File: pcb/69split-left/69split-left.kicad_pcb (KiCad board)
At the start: 2 copper layers, 157.5 x 108.9 mm, 96 parts, among them J1 USB_C_Receptacle_USB2.0_16P, J2 Conn_02x03_Odd_Even, J3 USB_C_Receptacle_USB2.0_16P, J4 Conn_01x09_Socket, SW1 SW_Push, SW10 SW_Push, SW11 SW_Push, SW12 SW_Push, SW13 SW_Push, SW14 SW_Push, SW15 SW_Push, SW16 SW_Push, SW17 SW_Push, SW18 SW_Push, SW19 SW_Push, SW2 SW_Push, SW20 SW_Push, SW21 SW_Push, SW22 SW_Push, SW23 SW_Push, SW24 SW_Push, SW25 SW_Push, SW26 SW_Push, SW27 SW_Push, SW28 SW_Push, SW29 SW_Push, SW3 SW_Push, SW30 SW_Push, SW31 SW_Push, SW32 SW_SPDT, SW4 SW_Push, SW5 SW_Push, SW6 SW_Push, SW7 SW_Push, SW8 SW_Push, SW9 SW_Push, U1 ATmega32U4-AU, U2 TLV76133DCY, U3 TPD2E2U06DCK, Y1 Crystal

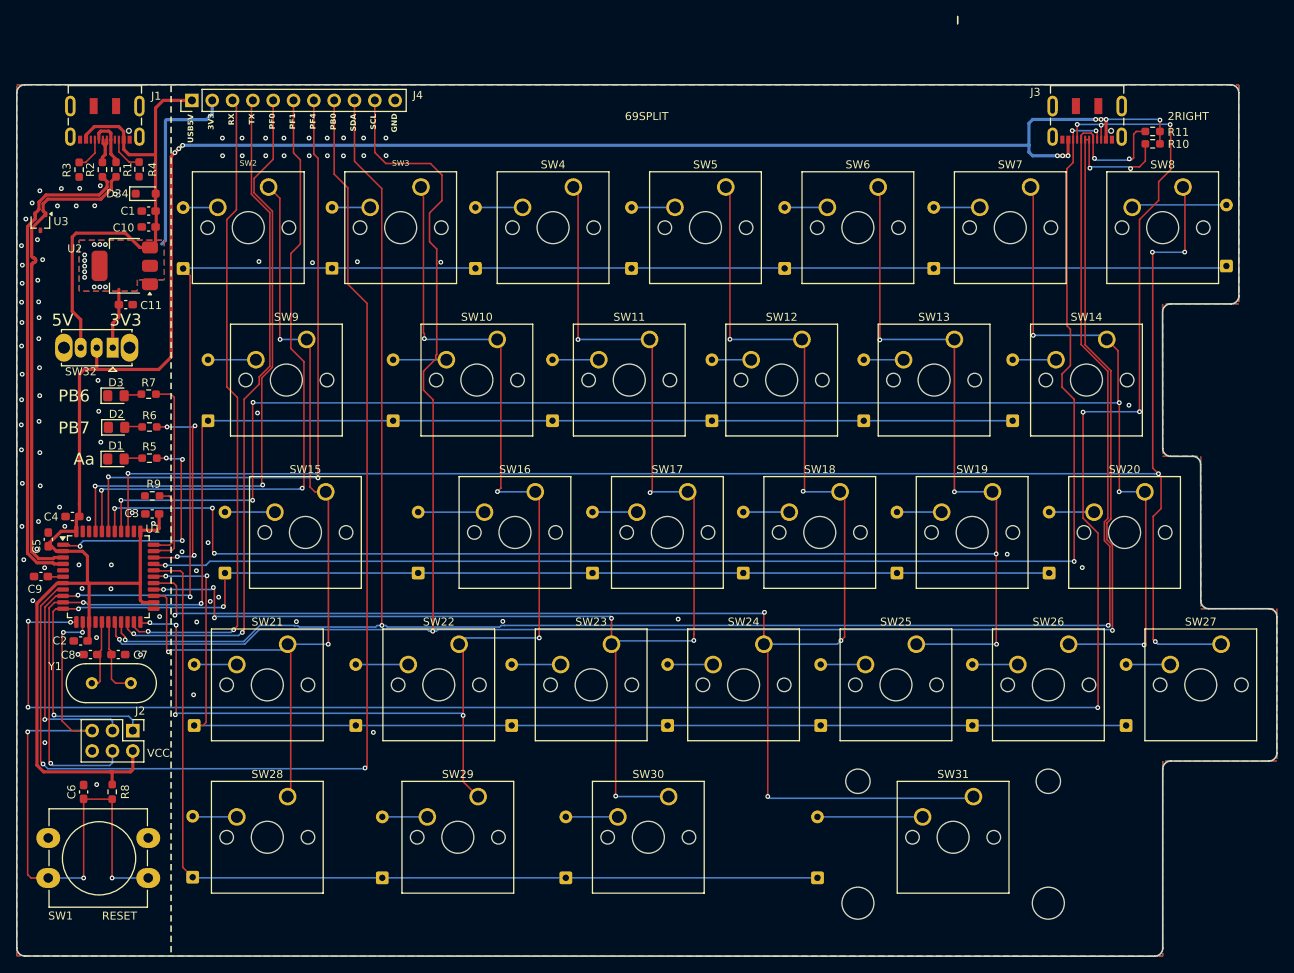
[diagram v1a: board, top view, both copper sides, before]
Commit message: Ordered the PCBs and parts!
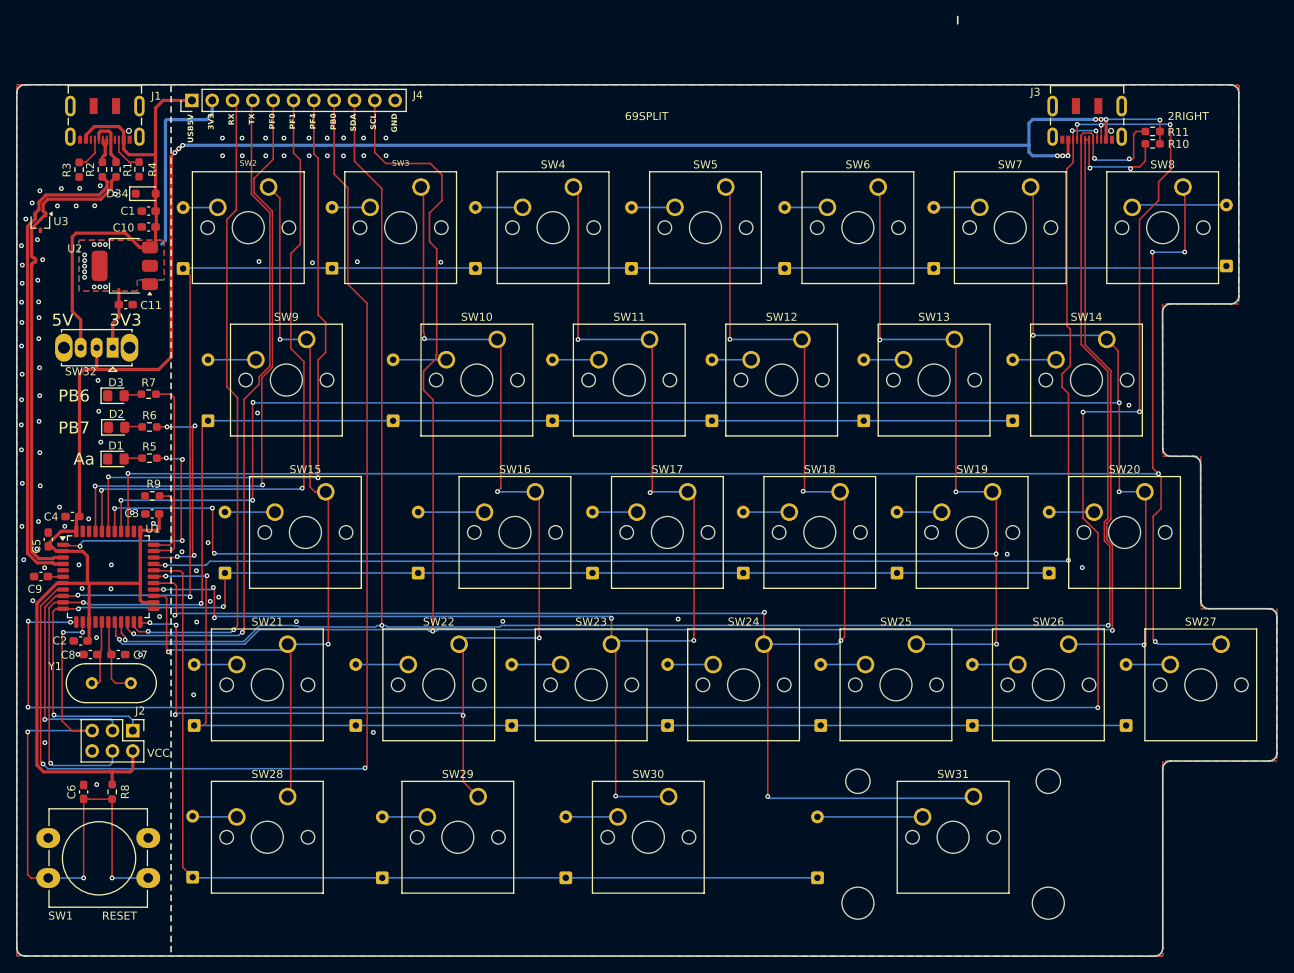
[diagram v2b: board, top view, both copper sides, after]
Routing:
- net /ATmega32U4/GPIO_OUT_PB6: track 175.0 -> 173.9 mm
- net /ATmega32U4/ADC4: track 80.5 -> 81.3 mm
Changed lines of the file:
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@@
 	)
 	(gr_line
-		(start 60.61 34.237091)
-		(end 211.36 34.237091)
+		(start 60.61 34.24)
+		(end 211.36 34.24)
 		(stroke
 			(width 0.2)
@@
 	)
 	(gr_arc
-		(start 59.61 35.237091)
-		(mid 59.902896 34.53)
-		(end 60.61 34.237091)
+		(start 59.6129 35.237091)
+		(mid 59.904947 34.532041)
+		(end 60.61 34.24)
 		(stroke
 			(width 0.2)
@@
 	)
 	(gr_line
-		(start 212.36 35.24)
+		(start 212.36 35.239623)
 		(end 212.369579 60.629579)
 		(stroke
@@
 		(layer "Dwgs.User")
 		(pts
-			(xy 60 143.14) (xy 59.902896 34.25)
+			(xy 59.81 143.140085) (xy 60.49 34.24)
 		)
-		(height -3.71)
+		(height -3.7)
 		(orientation 1)
 		(format
@@
 			(keep_text_aligned yes)
 		)
-		(gr_text "108.89 mm"
-			(at 55.14 88.695 90)
+		(gr_text "108.90 mm"
+			(at 54.96 88.690042 90)
 			(layer "Dwgs.User")
 			(effects
@@
 	)
 	(segment
+		(start 97.260715 83.370715)
+		(end 97.260715 68.639285)
+		(width 0.2)
+		(layer "F.Cu")
+		(net 54)
+	)
+	(segment
+		(start 97.260715 68.639285)
+		(end 98.21 67.69)
+		(width 0.2)
+		(layer "F.Cu")
+		(net 54)
+	)
+	(segment
+		(start 97.26 43.42)
+		(end 96.74 42.9)
+		(width 0.2)
+		(layer "F.Cu")
+		(net 54)
+	)
+	(segment
 		(start 71.06 83.539)
 		(end 71.06 90.0575)
@@
 	)
 	(segment
-		(start 96.74 42.9)
-		(end 96.74 36.19)
+		(start 98.21 63.93)
+		(end 97.26 62.98)
 		(width 0.2)
 		(layer "F.Cu")
@@
 	)
 	(segment
-		(start 97.260715 43.420715)
-		(end 96.74 42.9)
+		(start 98.21 67.69)
+		(end 98.21 63.93)
+		(width 0.2)
+		(layer "F.Cu")
+		(net 54)
+	)
+	(segment
+		(start 96.74 42.9)
+		(end 96.74 36.19)
 		(width 0.2)
 		(layer "F.Cu")
@@
 	)
 	(segment
-		(start 97.260715 83.370715)
-		(end 97.260715 43.420715)
+		(start 97.26 62.98)
+		(end 97.26 43.42)
 		(width 0.2)
 		(layer "F.Cu")
@@
 	)
 	(segment
-		(start 190.26 70.39)
-		(end 191.31 69.34)
+		(start 76.8825 94.3)
+		(end 76.7125 94.13)
 		(width 0.2)
 		(layer "F.Cu")
@@
 	)
 	(segment
-		(start 191.65 43.96028)
-		(end 191.65 41.1)
+		(start 191.61 39.97)
+		(end 191.65 40.01)
 		(width 0.2)
 		(layer "F.Cu")
@@
 	)
 	(segment
-		(start 76.8825 94.3)
-		(end 76.7125 94.13)
+		(start 190.26 72.03)
+		(end 190.26 70.39)
 		(width 0.2)
 		(layer "F.Cu")
@@
 	)
 	(segment
-		(start 191.61 39.97)
-		(end 191.65 40.01)
+		(start 191.65 40.01)
+		(end 191.65 41.1)
 		(width 0.2)
 		(layer "F.Cu")
@@
 	)
 	(segment
-		(start 191.31 69.34)
-		(end 191.31 64.79)
+		(start 191.54 39.97)
+		(end 191.61 39.97)
 		(width 0.2)
 		(layer "F.Cu")
@@
 	)
 	(segment
-		(start 191.65 40.01)
+		(start 191.65 43.96028)
 		(end 191.65 41.1)
 		(width 0.2)
@@
 	)
 	(segment
-		(start 191.78 73.55)
-		(end 190.26 72.03)
+		(start 194.51 39.99)
+		(end 194.65 40.13)
 		(width 0.2)
 		(layer "F.Cu")
@@
 	)
 	(segment
-		(start 190.88 64.36)
-		(end 190.88 44.73028)
+		(start 191.31 64.79)
+		(end 190.88 64.36)
 		(width 0.2)
 		(layer "F.Cu")
@@
 	)
 	(segment
-		(start 191.54 39.97)
-		(end 191.61 39.97)
+		(start 191.31 69.34)
+		(end 191.31 64.79)
 		(width 0.2)
 		(layer "F.Cu")
@@
 	)
 	(segment
-		(start 194.51 39.99)
-		(end 194.65 40.13)
+		(start 191.07 72.84)
+		(end 190.26 72.03)
 		(width 0.2)
 		(layer "F.Cu")
@@
 	)
 	(segment
-		(start 190.26 72.03)
-		(end 190.26 70.39)
+		(start 190.88 64.36)
+		(end 190.88 44.73028)
 		(width 0.2)
 		(layer "F.Cu")
@@
 	)
 	(segment
-		(start 191.31 64.79)
-		(end 190.88 64.36)
+		(start 194.65 40.13)
+		(end 194.65 41.1)
 		(width 0.2)
 		(layer "F.Cu")
@@
 	)
 	(segment
-		(start 190.88 44.73028)
-		(end 191.65 43.96028)
+		(start 191.07 93.68)
+		(end 191.07 72.84)
 		(width 0.2)
 		(layer "F.Cu")
@@
 	)
 	(segment
-		(start 194.65 40.13)
-		(end 194.65 41.1)
+		(start 190.26 70.39)
+		(end 191.31 69.34)
 		(width 0.2)
 		(layer "F.Cu")
@@
 	)
 	(segment
-		(start 191.78 93.82)
-		(end 191.78 73.55)
+		(start 190.88 44.73028)
+		(end 191.65 43.96028)
 		(width 0.2)
 		(layer "F.Cu")
@@
 	)
 	(via
-		(at 191.78 93.82)
+		(at 191.07 93.68)
 		(size 0.6)
 		(drill 0.3)
@@
 	(segment
 		(start 83.246 94.3)
-		(end 83.746 93.8)
+		(end 78.17 94.3)
 		(width 0.2)
 		(layer "B.Cu")
@@
 	)
 	(segment
-		(start 83.746 93.8)
-		(end 191.76 93.8)
+		(start 191.07 93.68)
+		(end 190.95 93.8)
 		(width 0.2)
 		(layer "B.Cu")
@@
 	)
 	(segment
-		(start 78.17 94.3)
+		(start 83.746 93.8)
 		(end 83.246 94.3)
 		(width 0.2)
@@
 	)
 	(segment
-		(start 191.76 93.8)
-		(end 191.78 93.82)
+		(start 190.95 93.8)
+		(end 83.746 93.8)
 		(width 0.2)
 		(layer "B.Cu")
@@
 	)
 	(segment
+		(start 176.99 66.24925)
+		(end 176.80775 66.067)
+		(width 0.2)
+		(layer "F.Cu")
+		(net 62)
+	)
+	(segment
 		(start 167.49 66.13)
 		(end 167.49 47.22425)
@@
 	)
 	(segment
-		(start 176.80775 85.117)
-		(end 176.80775 66.067)
-		(width 0.2)
-		(layer "F.Cu")
-		(net 62)
-	)
-	(segment
 		(start 84.119 87.15)
 		(end 84.09 87.179)
@@
 	)
 	(segment
+		(start 176.99 85.117)
+		(end 176.99 66.24925)
+		(width 0.2)
+		(layer "F.Cu")
+		(net 62)
+	)
+	(segment
 		(start 182.03 92.88)
 		(end 182.01 92.88)
@@
 	)
 	(via
-		(at 176.80775 85.117)
+		(at 176.99 85.117)
 		(size 0.6)
 		(drill 0.3)
@@
 	)
 	(segment
-		(start 181.57025 85.117)
-		(end 176.80775 85.117)
+		(start 182.08 104.17)
+		(end 182.077 104.167)
 		(width 0.2)
 		(layer "B.Cu")
@@
 	)
 	(segment
-		(start 182.08 104.17)
-		(end 182.077 104.167)
+		(start 181.57025 85.117)
+		(end 176.99 85.117)
 		(width 0.2)
 		(layer "B.Cu")
